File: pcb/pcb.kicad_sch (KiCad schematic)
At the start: 0 parts

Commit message: added symbols to schematic
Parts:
- added J1: Conn_01x16_Socket, Connector_PinHeader_1.00mm:PinHeader_1x16_P1.00mm_Vertical, symbol Connector:Conn_01x16_Socket
- added U1: W65C02SxP, Package_DIP:DIP-40_W15.24mm_Socket, symbol PCM_65xx-library:W65C02SxP
- added U2: W65C22SxP, Package_DIP:DIP-40_W15.24mm_Socket, symbol PCM_65xx-library:W65C22SxP
- added U3: 28C256, Package_DIP:DIP-28_W15.24mm_Socket, symbol Memory_EEPROM:28C256
- added U4: HM62256BLP, Package_DIP:DIP-28_W15.24mm_Socket, symbol Memory_RAM:HM62256BLP

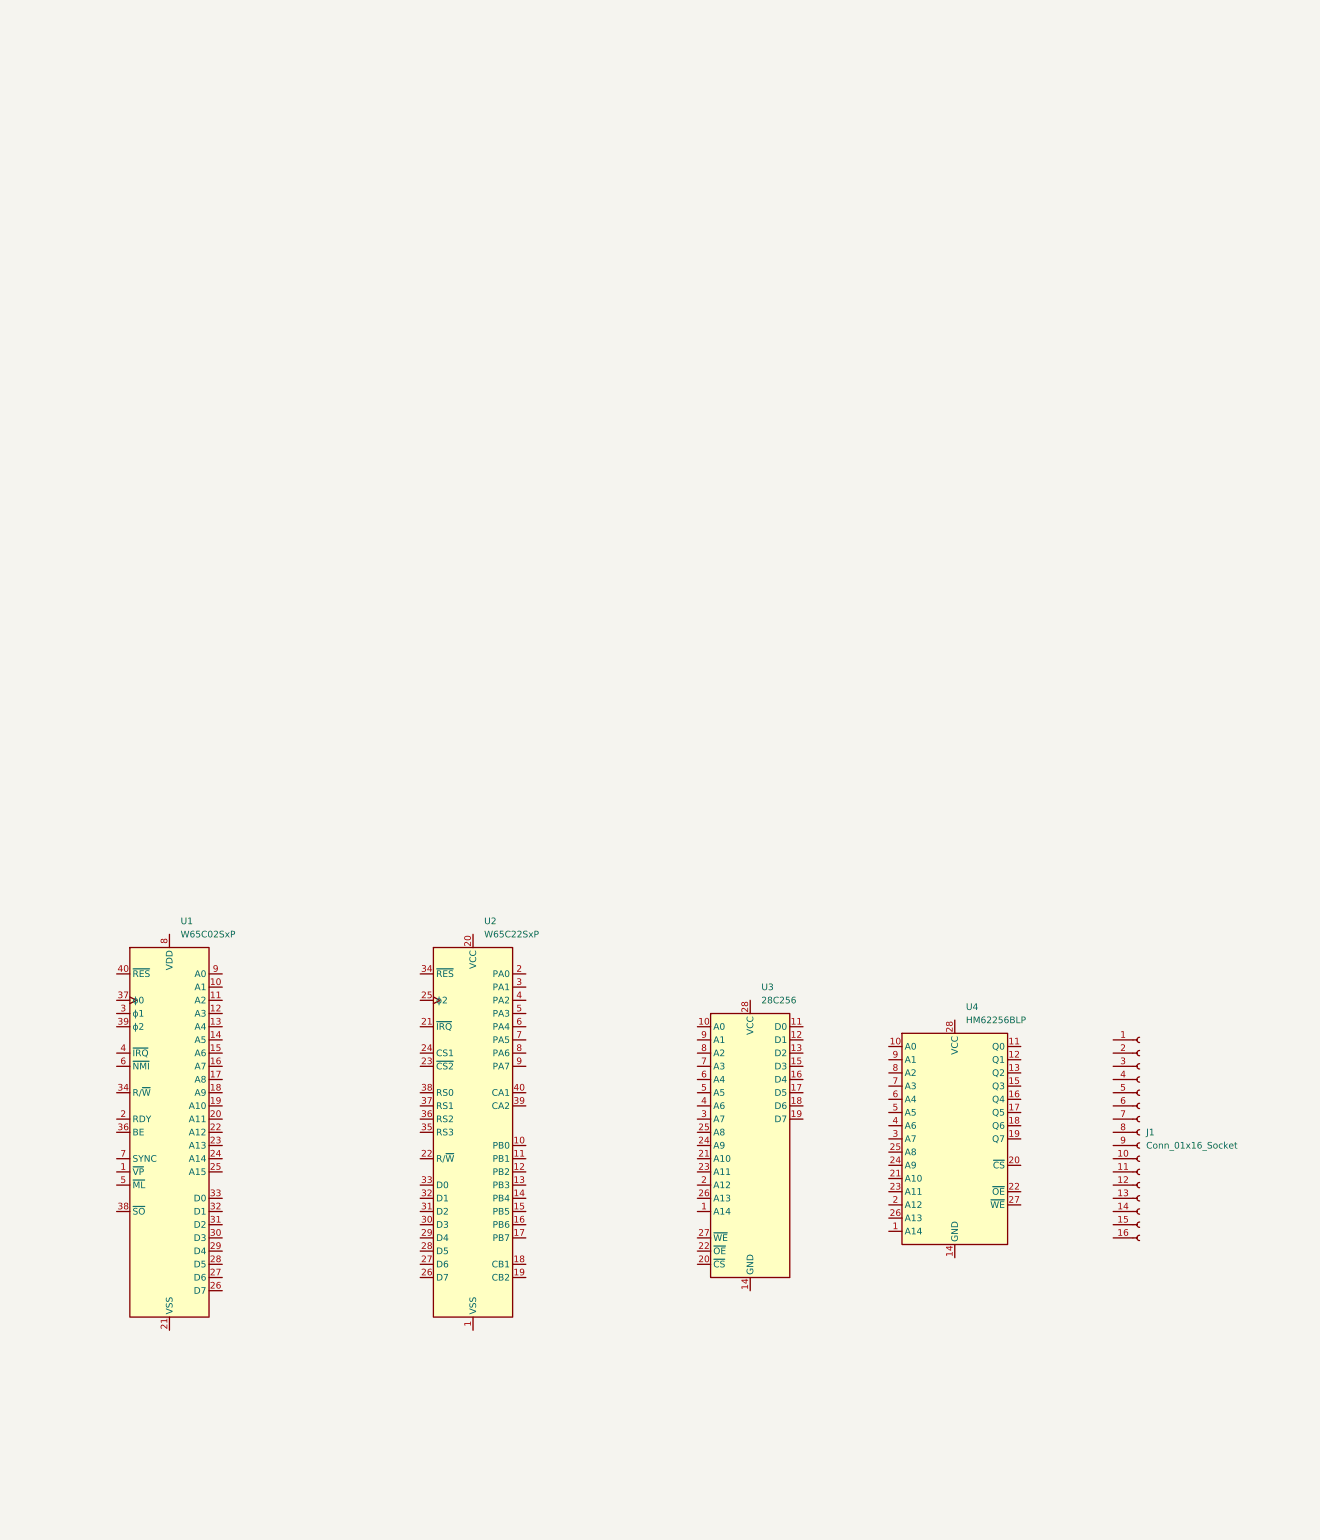
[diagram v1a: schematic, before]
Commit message: update
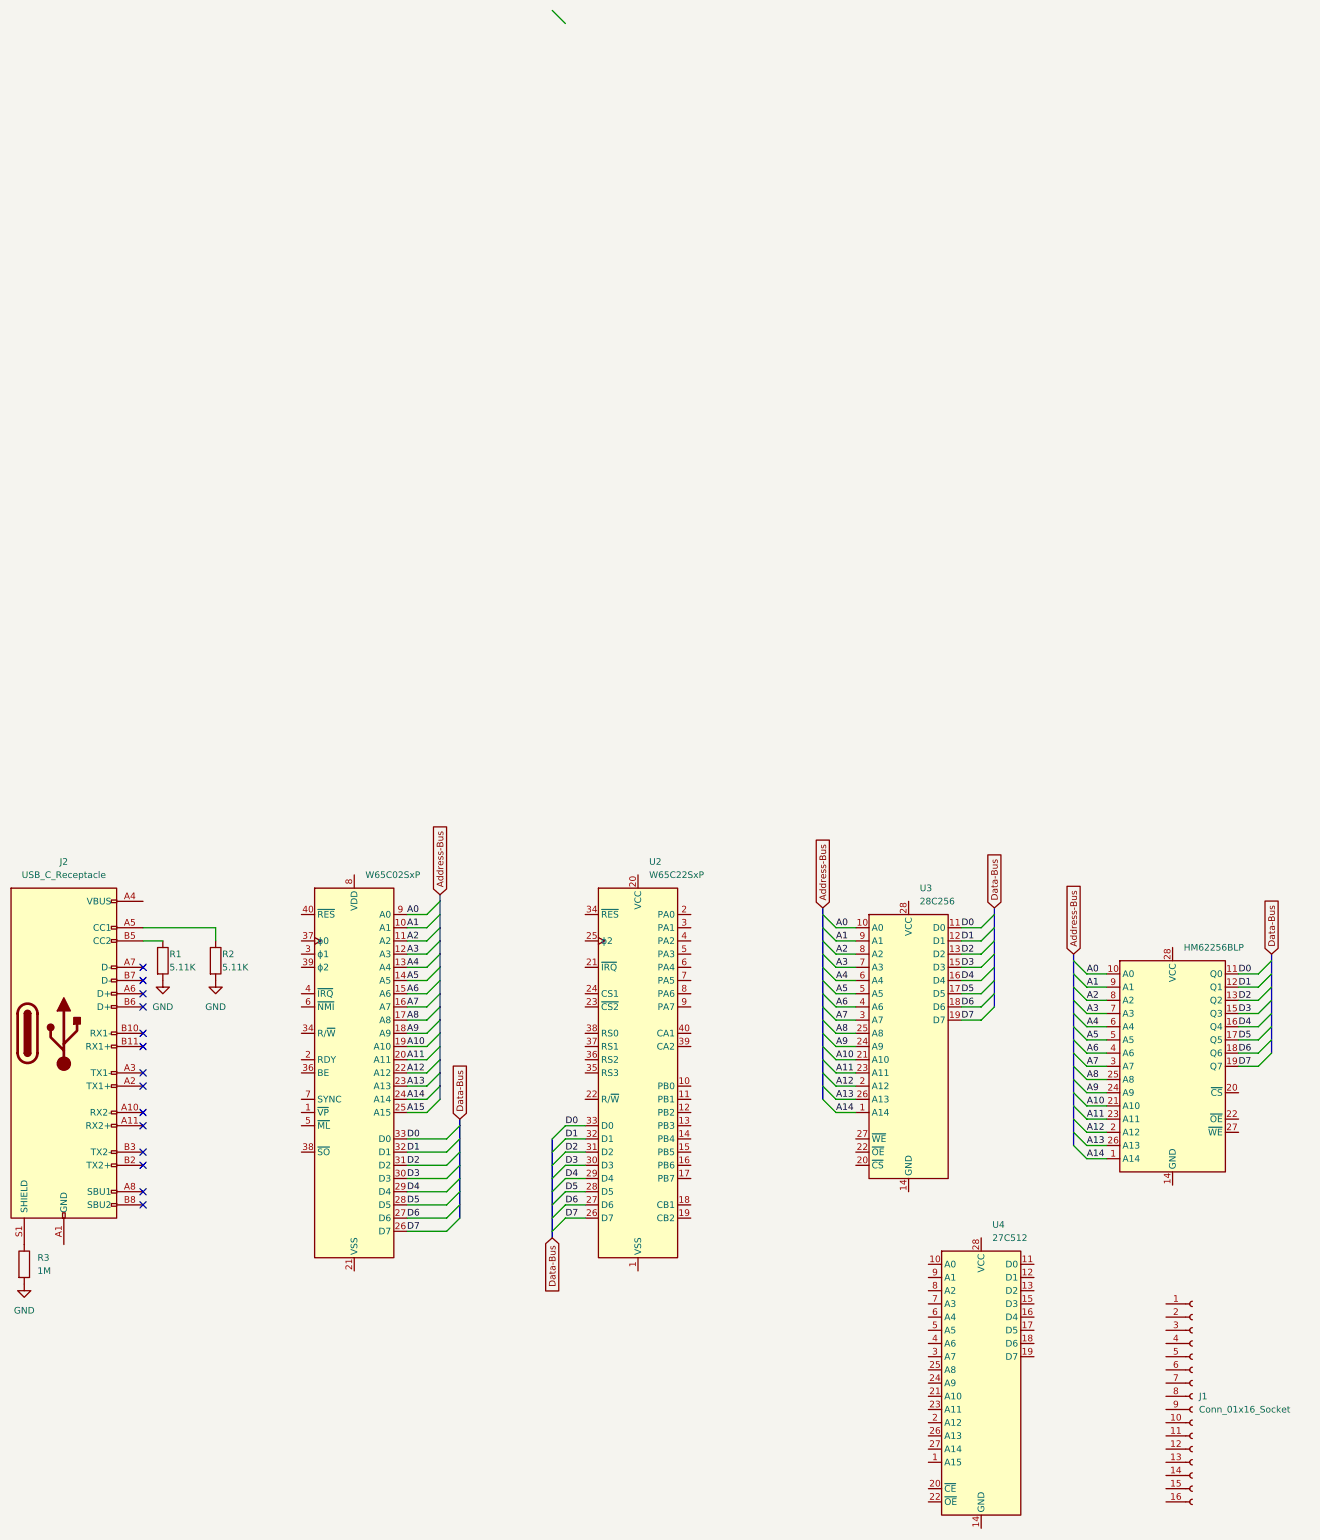
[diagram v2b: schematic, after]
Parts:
- added J2: USB_C_Receptacle, Connector_USB:USB_C_Receptacle_Amphenol_12401548E4-2A, symbol Connector:USB_C_Receptacle
- added R1, R2: 5.11K, symbol Device:R
- added R3: 1M, symbol Device:R
- added U4: 27C512, Package_DIP:DIP-28_W15.24mm_Socket, symbol Memory_EPROM:27C512
- renumbered U4 to U5
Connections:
- net A1: now reaches U1.10 (A1)
- net A1: now also U3.9 (A1), U5.9 (A1)
- net A2: now reaches U1.11 (A2)
- net A2: now also U3.8 (A2), U5.8 (A2)
- net A3: now reaches U1.12 (A3)
- net A3: now also U3.7 (A3), U5.7 (A3)
- net A4: now reaches U1.13 (A4)
- net A4: now also U3.6 (A4), U5.6 (A4)
- net A5: now reaches U1.14 (A5)
- net A5: now also U3.5 (A5), U5.5 (A5)
- net A6: now reaches U1.15 (A6)
- net A6: now also U3.4 (A6), U5.4 (A6)
- net A7: now reaches U1.16 (A7)
- net A7: now also U3.3 (A7), U5.3 (A7)
- net A8: now reaches U1.17 (A8)
- net A8: now also U3.25 (A8), U5.25 (A8)
- net A9: now reaches U1.18 (A9)
- net A9: now also U3.24 (A9), U5.24 (A9)
- net A10: now reaches U1.19 (A10)
- net A10: now also U3.21 (A10), U5.21 (A10)
- net A11: now reaches U1.20 (A11)
- net A11: now also U3.23 (A11), U5.23 (A11)
- net A12: now reaches U1.22 (A12)
- net A12: now also U3.2 (A12), U5.2 (A12)
- net A13: now reaches U1.23 (A13)
- net A13: now also U3.26 (A13), U5.26 (A13)
- net A14: now reaches U1.24 (A14)
- net A14: now also U3.1 (A14), U5.1 (A14)
- net A15: now reaches U1.25 (A15)
- net D7: now reaches U1.26 (D7)
- net D7: now also U2.26 (D7), U3.19 (D7), U5.19 (Q7)
- net D6: now reaches U1.27 (D6)
- net D6: now also U2.27 (D6), U3.18 (D6), U5.18 (Q6)
- net D5: now reaches U1.28 (D5)
- net D5: now also U2.28 (D5), U3.17 (D5), U5.17 (Q5)
- net D4: now reaches U1.29 (D4)
- net D4: now also U2.29 (D4), U3.16 (D4), U5.16 (Q4)
- net D3: now reaches U1.30 (D3)
- net D3: now also U2.30 (D3), U3.15 (D3), U5.15 (Q3)
- net D2: now reaches U1.31 (D2)
- net D2: now also U2.31 (D2), U3.13 (D2), U5.13 (Q2)
- net D1: now reaches U1.32 (D1)
- net D1: now also U2.32 (D1), U3.12 (D1), U5.12 (Q1)
- net D0: now reaches U1.33 (D0)
- net D0: now also U2.33 (D0), U3.11 (D0), U5.11 (Q0)
- net A0: now reaches U1.9 (A0)
- net A0: now also U3.10 (A0), U5.10 (A0)
- new net: J2.A1 (GND), J2.A12 (GND), J2.B1 (GND), J2.B12 (GND)
- new net: J2.A4 (VBUS), J2.A9 (VBUS), J2.B4 (VBUS), J2.B9 (VBUS)
- new net: J2.A5 (CC1), R2.1
- new net: J2.B5 (CC2), R1.1
- new net: J2.S1 (SHIELD), R3.1
- new net GND: R1.2, R2.2, R3.2
- no-connect marks 0 -> 14
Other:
- moved on the sheet: J1, U2, U3

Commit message: lots of updates
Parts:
- removed J1: Conn_01x16_Socket, Connector_PinHeader_1.00mm:PinHeader_1x16_P1.00mm_Vertical, symbol Connector:Conn_01x16_Socket
- removed J2: USB_C_Receptacle, Connector_USB:USB_C_Receptacle_Amphenol_12401548E4-2A, symbol Connector:USB_C_Receptacle
- removed U4: 27C512, Package_DIP:DIP-28_W15.24mm_Socket, symbol Memory_EPROM:27C512
- added J1: USB_C_Receptacle, Connector_USB:USB_C_Receptacle_Amphenol_12401548E4-2A, symbol Connector:USB_C_Receptacle
- added J2, J3, J4, J5: Conn_01x10_Pin, Connector_PinHeader_2.00mm:PinHeader_1x10_P2.00mm_Vertical, symbol Connector:Conn_01x10_Pin
- added J6: Conn_01x02_Pin, Connector_PinHeader_2.00mm:PinHeader_1x02_P2.00mm_Vertical, symbol Connector:Conn_01x02_Pin
- added R4: 1M, Resistor_THT:R_Axial_DIN0207_L6.3mm_D2.5mm_P7.62mm_Horizontal, symbol Device:R
- added SW1: SW_Push, Button_Switch_THT:SW_PUSH-12mm, symbol Switch:SW_Push
- added U10: 74HC04, Package_DIP:DIP-14_W7.62mm_Socket, symbol 74xx:74LS04
- added U3: W65C22SxP, Package_DIP:DIP-40_W15.24mm_Socket, symbol PCM_65xx-library:W65C22SxP
- added U6: 74HC684, Package_DIP:DIP-20_W7.62mm_Socket, symbol Other:74HC684
- added U7, U8: 74HC680, Package_DIP:DIP-20_W7.62mm_Socket, symbol Other:74HC680
- added U9: 74HC00, Package_DIP:DIP-14_W7.62mm_Socket, symbol 74xx:74LS00
- added Y1: MCO-1510A, Oscillator:Oscillator_DIP-14, symbol Other:MCO-1510A
- R1: value 5.11K -> 220; footprint (none) -> Resistor_THT:R_Axial_DIN0207_L6.3mm_D2.5mm_P7.62mm_Horizontal
- R2: footprint (none) -> Resistor_THT:R_Axial_DIN0207_L6.3mm_D2.5mm_P7.62mm_Horizontal
- R3: value 1M -> 5.11K; footprint (none) -> Resistor_THT:R_Axial_DIN0207_L6.3mm_D2.5mm_P7.62mm_Horizontal
- renumbered U3 to U4
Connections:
- net A0: now also U2.38 (RS0), U3.38 (RS0)
- net A1: now also U2.37 (RS1), U3.37 (RS1)
- net A10: now also U6.6 (P2), U7.3 (A2), U8.4 (A3)
- net A11: now also U6.8 (P3), U7.4 (A3), U8.5 (A4)
- net A12: now also U6.11 (P4), U7.5 (A4), U8.6 (A5)
- net A13: now also U6.13 (P5), U7.6 (A5), U8.7 (A6)
- net A14: now also U6.15 (P6), U7.7 (A6), U8.8 (A7)
- net A15: now also U10.1, U6.17 (P7), U7.13 (A11), U8.13 (A11)
- net A2: now also U2.36 (RS2), U3.36 (RS2)
- net A3: now also U2.35 (RS3), U3.35 (RS3)
- net A4: now also U7.8 (A7), U8.1 (A0)
- net A5: now also U7.9 (A8), U8.9 (A8)
- net A6: now also U7.11 (A9), U8.11 (A9)
- net A7: now also U7.12 (A10), U8.12 (A10)
- net A8: now also U6.2 (P0), U7.1 (A0), U8.2 (A1)
- net A9: now also U6.4 (P1), U7.2 (A1), U8.3 (A2)
- net D0: now also U3.33 (D0)
- net D1: now also U3.32 (D1)
- net D2: now also U3.31 (D2)
- net D3: now also U3.30 (D3)
- net D4: now also U3.29 (D4)
- net D5: now also U3.28 (D5)
- net D6: now also U3.27 (D6)
- net D7: now also U3.26 (D7)
- net GND: now also U1.21 (VSS), U2.1 (VSS), U4.14 (GND), U4.22 (~{OE}), U5.14 (GND), U5.22 (~{OE}), J1.A1 (GND), J1.A12 (GND), J1.B1 (GND), J1.B12 (GND), J6.2 (Pin_2), R4.2, SW1.1, U10.7 (GND), U3.1 (VSS), U6.10 (GND), U6.18 (Q7), U7.10 (VSS), U7.17 (P3), U7.19 (C), U8.10 (VSS), U8.14 (P0), U8.15 (P1), U8.16 (P2), U8.19 (C), U9.7 (GND), Y1.7 (GND); no longer R1.2
- net at R2.1: now also J1.B5 (CC2)
- net +5V: now reaches R1.1
- net +5V: now also U1.2 (RDY), U1.36 (BE), U1.38 (~{SO}), U1.6 (~{NMI}), U1.8 (VDD), U2.20 (VCC), U4.27 (~{WE}), U4.28 (VCC), U5.28 (VCC), J1.A4 (VBUS), J1.A9 (VBUS), J1.B4 (VBUS), J1.B9 (VBUS), J6.1 (Pin_1), U10.14 (VCC), U3.20 (VCC), U6.12 (Q4), U6.14 (Q5), U6.16 (Q6), U6.20 (VCC), U6.3 (Q0), U6.5 (Q1), U6.7 (Q2), U6.9 (Q3), U7.14 (P0), U7.15 (P1), U7.16 (P2), U7.20 (VCC), U8.17 (P3), U8.20 (VCC), U9.14 (VCC), Y1.14 (Vcc)
- net at R3.1: now also J1.A5 (CC1)
- net R/~{W}: now reaches U1.34 (R/~{W})
- net R/~{W}: now also U2.22 (R/~{W}), U5.27 (~{WE}), U3.22 (R/~{W})
- net CLK: now reaches U1.37 (ϕ0)
- net CLK: now also U2.25 (ϕ2), U3.25 (ϕ2), U9.2, Y1.8 (OUT)
- net at U1.4 (~{IRQ}): now also U9.8
- net ~{RES}: now reaches U1.40 (~{RES})
- net ~{RES}: now also R1.2, U2.34 (~{RES}), SW1.2, U3.34 (~{RES})
- net at U4.20 (~{CS}): now also U10.2
- net at U5.20 (~{CS}): now also U9.3
- net at U2.10 (PB0): now also J3.1 (Pin_1)
- net at U2.11 (PB1): now also J3.2 (Pin_2)
- net at U2.12 (PB2): now also J3.3 (Pin_3)
- net at U2.13 (PB3): now also J3.4 (Pin_4)
- net at U2.14 (PB4): now also J3.5 (Pin_5)
- net at U2.15 (PB5): now also J3.6 (Pin_6)
- net at U2.16 (PB6): now also J3.7 (Pin_7)
- net at U2.17 (PB7): now also J3.8 (Pin_8)
- net at U2.18 (CB1): now also J3.9 (Pin_9)
- net at U2.19 (CB2): now also J3.10 (Pin_10)
- net at U2.2 (PA0): now also J2.1 (Pin_1)
- net ~{IRQ} 1: now reaches U2.21 (~{IRQ})
- net ~{IRQ} 1: now also U9.4
- net at U2.23 (~{CS2}): now also U10.5, U7.18 (Y)
- net at U2.24 (CS1): now also U10.6
- net at U2.3 (PA1): now also J2.2 (Pin_2)
- net at U2.39 (CA2): now also J2.10 (Pin_10)
- net at U2.4 (PA2): now also J2.3 (Pin_3)
- net at U2.40 (CA1): now also J2.9 (Pin_9)
- net at U2.5 (PA3): now also J2.4 (Pin_4)
- net at U2.6 (PA4): now also J2.5 (Pin_5)
- net at U2.7 (PA5): now also J2.6 (Pin_6)
- net at U2.8 (PA6): now also J2.7 (Pin_7)
- net at U2.9 (PA7): now also J2.8 (Pin_8)
- new net: J5.1 (Pin_1), U3.10 (PB0)
- new net: J5.2 (Pin_2), U3.11 (PB1)
- new net: J5.3 (Pin_3), U3.12 (PB2)
- new net: J5.4 (Pin_4), U3.13 (PB3)
- new net: J5.5 (Pin_5), U3.14 (PB4)
- new net: J5.6 (Pin_6), U3.15 (PB5)
- new net: J5.7 (Pin_7), U3.16 (PB6)
- new net: J5.8 (Pin_8), U3.17 (PB7)
- new net: J5.9 (Pin_9), U3.18 (CB1)
- new net: J5.10 (Pin_10), U3.19 (CB2)
- new net: J4.1 (Pin_1), U3.2 (PA0)
- new net: U10.9, U3.23 (~{CS2}), U8.18 (Y)
- new net: U10.8, U3.24 (CS1)
- new net: J4.2 (Pin_2), U3.3 (PA1)
- new net: J4.10 (Pin_10), U3.39 (CA2)
- new net: J4.3 (Pin_3), U3.4 (PA2)
- new net: J4.9 (Pin_9), U3.40 (CA1)
- new net: J4.4 (Pin_4), U3.5 (PA3)
- new net: J4.5 (Pin_5), U3.6 (PA4)
- new net: J4.6 (Pin_6), U3.7 (PA5)
- new net: J4.7 (Pin_7), U3.8 (PA6)
- new net: J4.8 (Pin_8), U3.9 (PA7)
- new net: J1.S1 (SHIELD), R4.1
- new net: U10.3, U6.1 (~{P>Q})
- new net: U10.4, U9.1
- new net: U9.10, U9.6, U9.9
- new net ~{IRQ} 2: U3.21 (~{IRQ}), U9.5
- no-connect marks 14 -> 20
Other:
- moved on the sheet: U2, U4
